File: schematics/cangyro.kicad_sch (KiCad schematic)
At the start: 14 parts, among them J1 Conn_01x06 CAN & PWR, J2 Conn_01x10 IMU BNO080, P1 USB_C_Plug_USB2.0 Serial, SW1 SW_Push IMU_RST, U1 STM32G474CBTx, U2 MCP2562-E-MF, U3 AP2112K-3.3

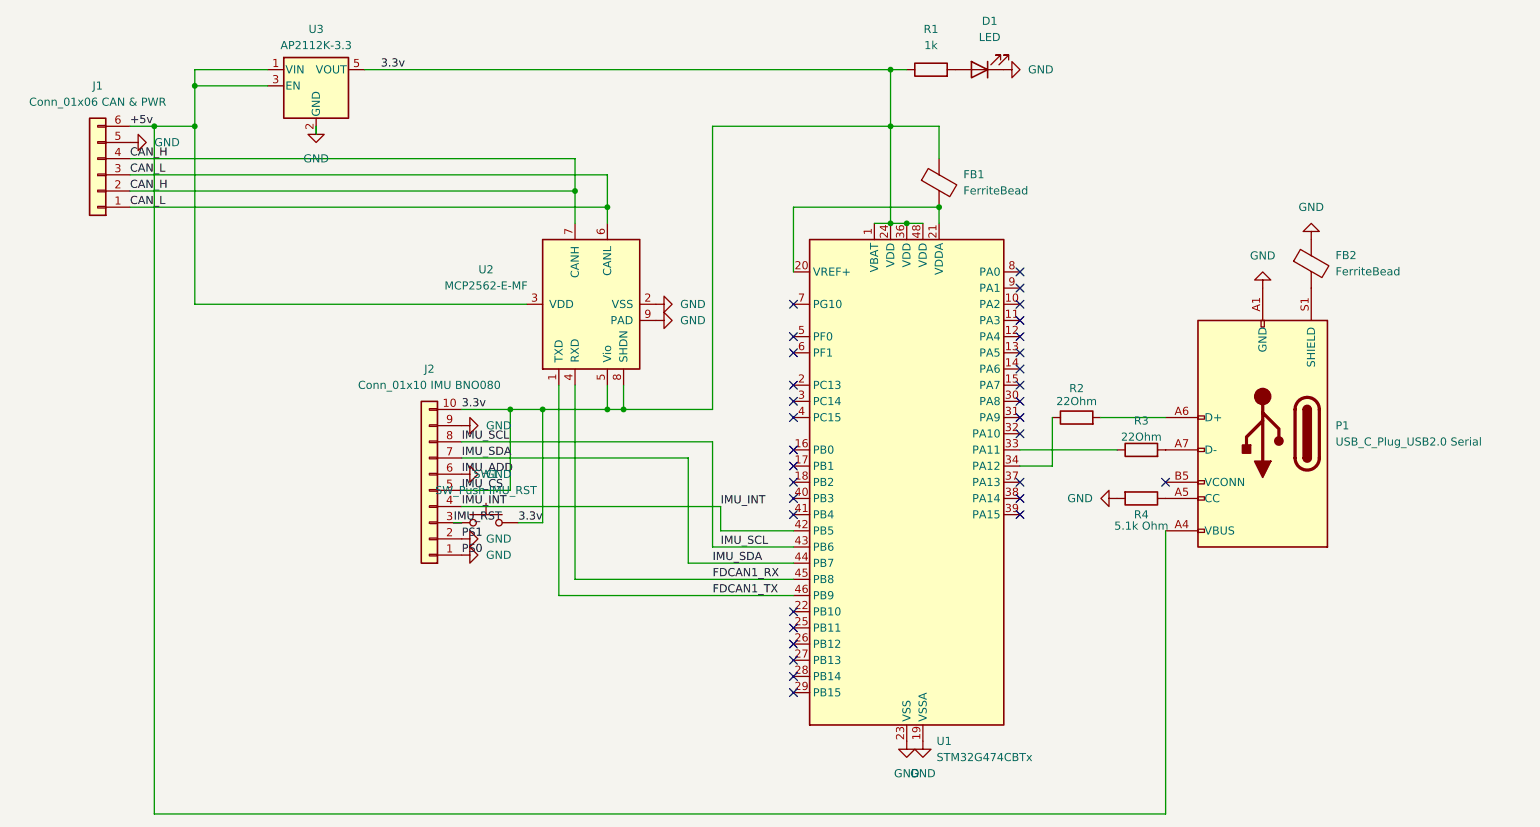
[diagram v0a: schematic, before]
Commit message: Base software project
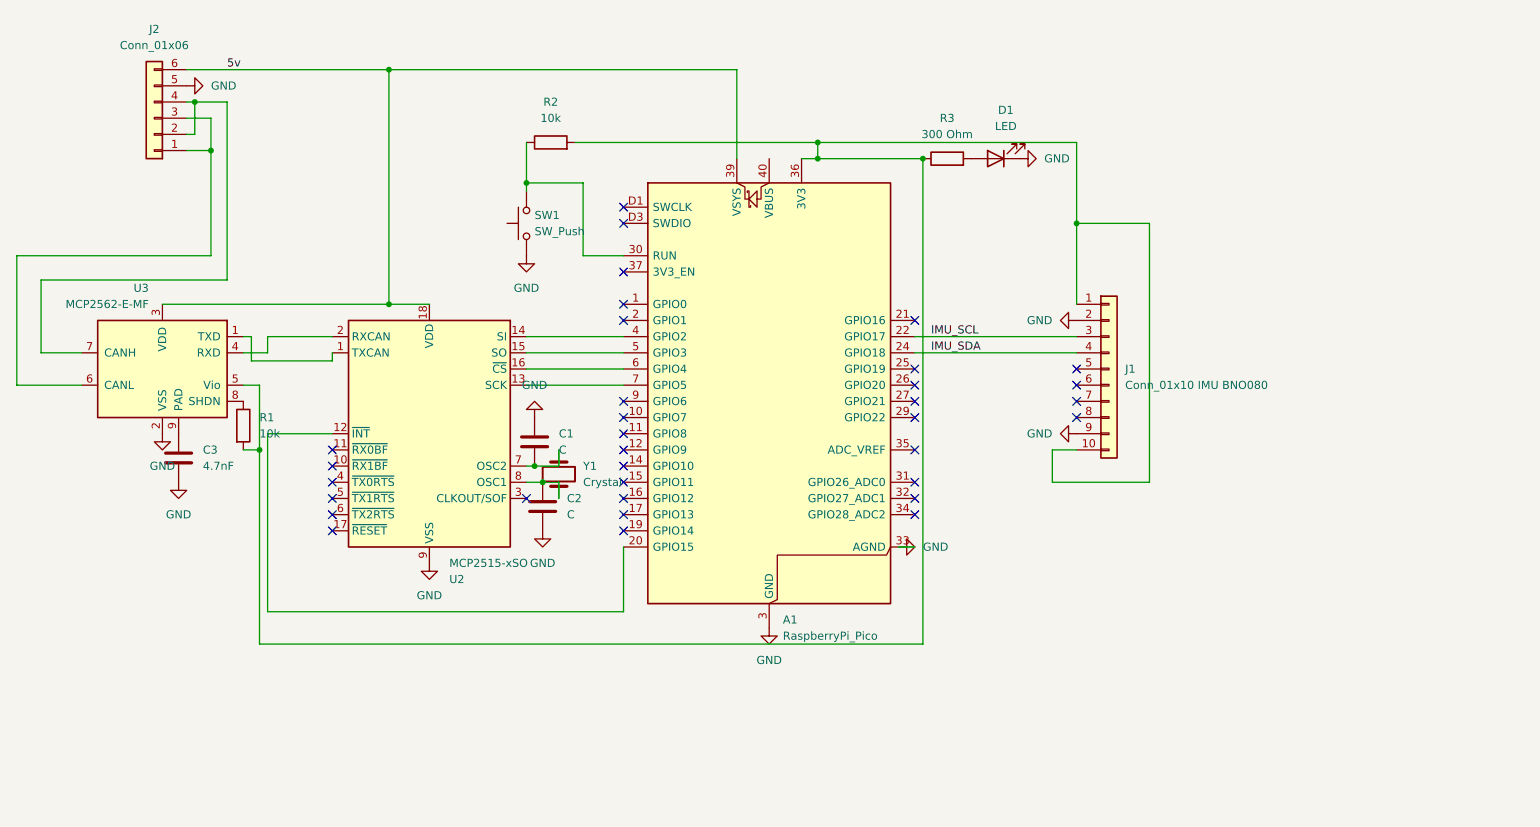
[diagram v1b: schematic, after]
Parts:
- removed FB1, FB2: FerriteBead, Inductor_SMD:L_0805_2012Metric, symbol Device:FerriteBead
- removed J1: Conn_01x06 CAN & PWR, TerminalBlock_Phoenix:TerminalBlock_Phoenix_MKDS-1,5-6-5.08_1x06_P5.08mm_Horizontal, symbol Connector_Generic:Conn_01x06
- removed J2: Conn_01x10 IMU BNO080, Connector_PinSocket_1.00mm:PinSocket_1x10_P1.00mm_Vertical, symbol Connector_Generic:Conn_01x10
- removed P1: USB_C_Plug_USB2.0 Serial, Connector_USB:USB_C_Receptacle_HRO_TYPE-C-31-M-17, symbol Connector:USB_C_Plug_USB2.0
- removed R4: 5.1k Ohm, Resistor_SMD:R_0805_2012Metric, symbol Device:R
- removed U1: STM32G474CBTx, Package_QFP:LQFP-48_7x7mm_P0.5mm, symbol MCU_ST_STM32G4:STM32G474CBTx
- removed U2: MCP2562-E-MF, Package_DFN_QFN:DFN-8-1EP_3x3mm_P0.65mm_EP1.55x2.4mm, symbol Interface_CAN_LIN:MCP2562-E-MF
- removed U3: AP2112K-3.3, Package_TO_SOT_SMD:SOT-23-5, symbol Regulator_Linear:AP2112K-3.3
- added A1: RaspberryPi_Pico, Module:RaspberryPi_Pico_SMD_HandSolder, symbol MCU_Module:RaspberryPi_Pico_Debug
- added C1, C2: C, symbol Device:C
- added C3: 4.7nF, symbol Device:C
- added J1: Conn_01x10 IMU BNO080, symbol Connector_Generic:Conn_01x10
- added J2: Conn_01x06, symbol Connector_Generic:Conn_01x06
- added U2: MCP2515-xSO, Package_SO:SOIC-18W_7.5x11.6mm_P1.27mm, symbol Interface_CAN_LIN:MCP2515-xSO
- added U3: MCP2562-E-MF, Package_DFN_QFN:DFN-8-1EP_3x3mm_P0.65mm_EP1.55x2.4mm, symbol Interface_CAN_LIN:MCP2562-E-MF
- added Y1: Crystal, symbol Device:Crystal
- D1: footprint LED_SMD:LED_0805_2012Metric -> (none)
- R1: value 1k -> 10k; footprint Resistor_SMD:R_0805_2012Metric -> (none)
- R2: value 22Ohm -> 10k; footprint Resistor_SMD:R_0805_2012Metric -> (none)
- R3: value 22Ohm -> 300 Ohm; footprint Resistor_SMD:R_0805_2012Metric -> (none)
- SW1: value SW_Push IMU_RST -> SW_Push; footprint Button_Switch_SMD:SW_SPST_TL3342 -> (none)
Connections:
- net IMU_RST is gone; now on net GND: SW1.1
- net GND: now also A1.13 (GND), A1.18 (GND), A1.23 (GND), A1.28 (GND), A1.3 (GND), A1.33 (AGND), A1.38 (GND), A1.8 (GND), A1.D2 (GND), C1.1, C2.2, C3.2, J1.2 (Pin_2), J1.9 (Pin_9), J2.5 (Pin_5), U2.9 (VSS), U3.2 (VSS)
- net IMU_SCL: now also A1.22 (GPIO17), J1.3 (Pin_3)
- net IMU_SDA: now also A1.24 (GPIO18), J1.4 (Pin_4)
- net at R1.2: now also R2.2, R3.1, A1.36 (3V3), J1.1 (Pin_1), J1.10 (Pin_10), U3.5 (Vio); no longer D1.2 (A)
- net at R3.2: now also D1.2 (A)
- net at R2.1: now also SW1.2, A1.30 (RUN)
- net 3.3v: no longer names the net of R1.1
- net 3.3v: now also U3.8 (SHDN); no longer SW1.2
- new net: U2.1 (TXCAN), U3.1 (TXD)
- new net: U2.2 (RXCAN), U3.4 (RXD)
- new net: J2.1 (Pin_1), J2.3 (Pin_3), U3.6 (CANL)
- new net: J2.2 (Pin_2), J2.4 (Pin_4), U3.7 (CANH)
- new net: C3.1, U3.9 (PAD)
- new net: C1.2, U2.7 (OSC2), Y1.2
- new net: A1.20 (GPIO15), U2.12 (~{INT})
- new net: A1.7 (GPIO5), U2.13 (SCK)
- new net: A1.4 (GPIO2), U2.14 (SI)
- new net: A1.5 (GPIO3), U2.15 (SO)
- new net: A1.6 (GPIO4), U2.16 (~{CS})
- new net: C2.1, U2.8 (OSC1), Y1.1
- new net 5v: A1.39 (VSYS), J2.6 (Pin_6), U2.18 (VDD), U3.3 (VDD)
- no-connect marks 32 -> 34
